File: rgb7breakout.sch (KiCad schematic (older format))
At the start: 8 parts

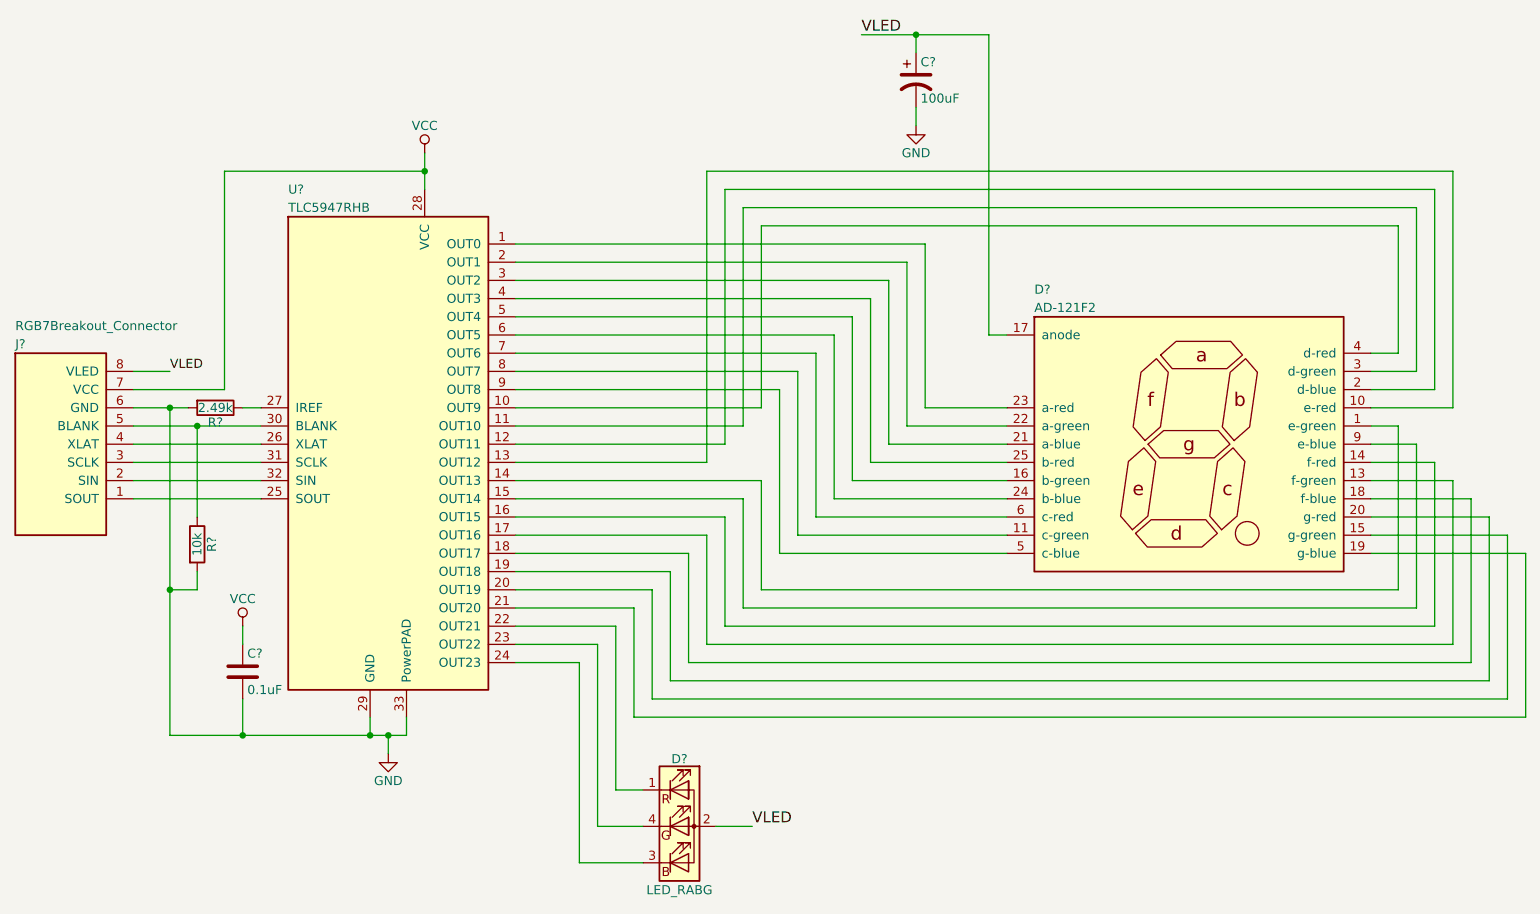
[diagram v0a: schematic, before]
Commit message: annotated components
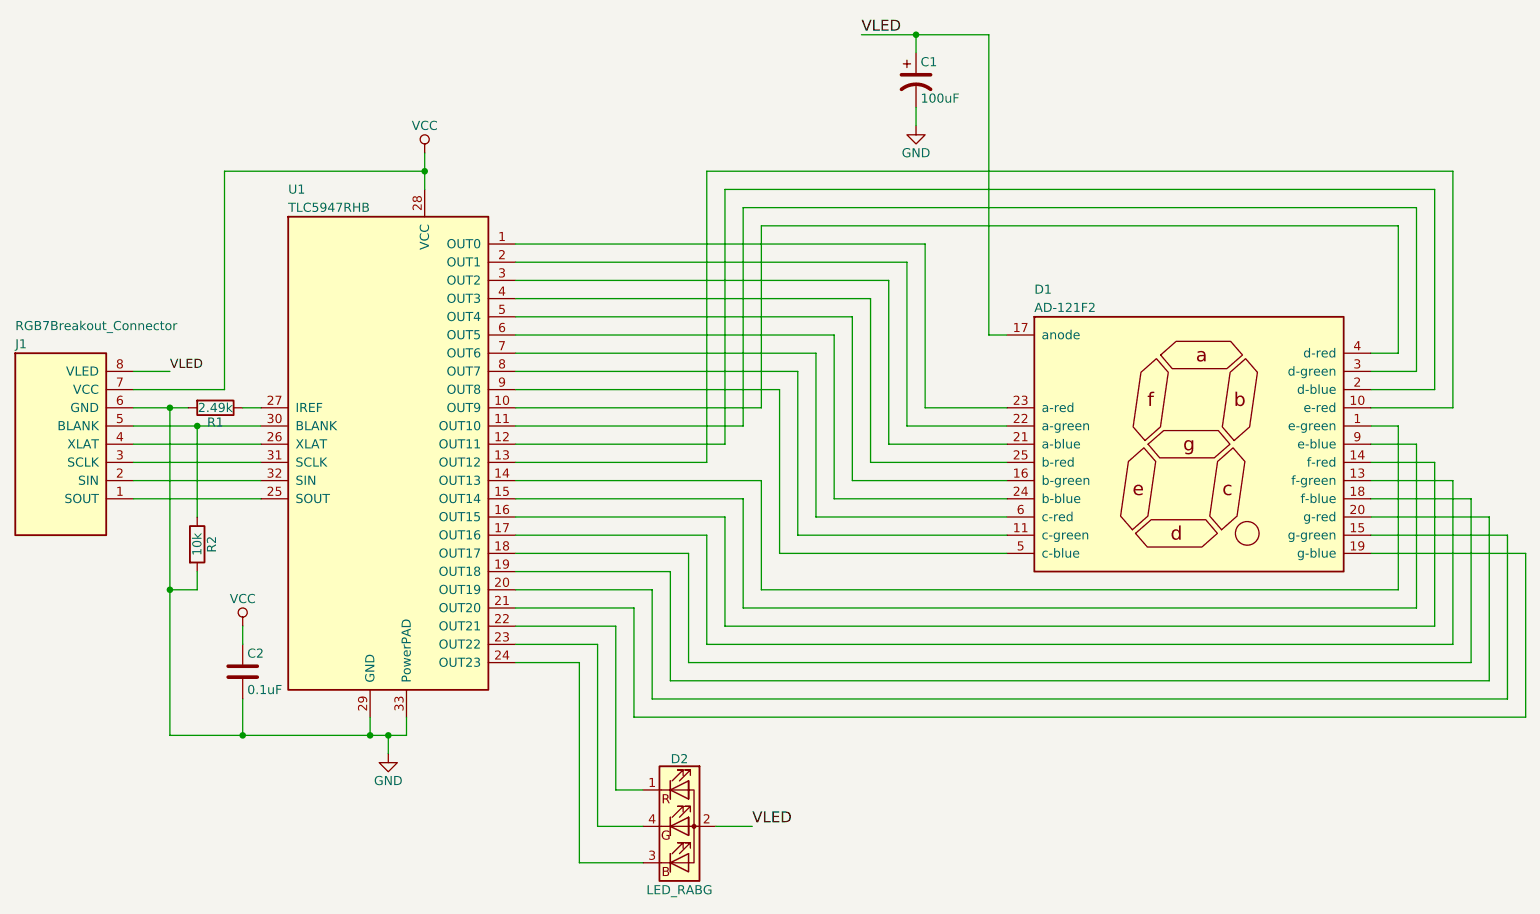
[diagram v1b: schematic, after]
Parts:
- gave numbers to parts that had none: 8
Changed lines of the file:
@@
 $EndDescr
 $Comp
-L AD-121F2 D?
+L AD-121F2 D1
 U 1 1 59B77441
 P 7900 3900
-F 0 "D?" H 7050 4750 50  0000 L CNN
+F 0 "D1" H 7050 4750 50  0000 L CNN
 F 1 "AD-121F2" H 7050 4650 50  0000 L CNN
 F 2 "" H 7900 3900 50  0001 C CNN
@@
 $EndComp
 $Comp
-L LED_RABG D?
+L LED_RABG D2
 U 1 1 59B77822
 P 5100 6000
-F 0 "D?" H 5100 6370 50  0000 C CNN
+F 0 "D2" H 5100 6370 50  0000 C CNN
 F 1 "LED_RABG" H 5100 5650 50  0000 C CNN
 F 2 "" H 5100 5950 50  0001 C CNN
@@
 $EndComp
 $Comp
-L VCC #PWR?
+L VCC #PWR2
 U 1 1 59B778E2
 P 3700 2300
-F 0 "#PWR?" H 3700 2150 50  0001 C CNN
+F 0 "#PWR2" H 3700 2150 50  0001 C CNN
 F 1 "VCC" H 3700 2450 50  0000 C CNN
 F 2 "" H 3700 2300 50  0001 C CNN
@@
 $EndComp
 $Comp
-L GND #PWR?
+L GND #PWR4
 U 1 1 59B77905
 P 3500 5600
-F 0 "#PWR?" H 3500 5350 50  0001 C CNN
+F 0 "#PWR4" H 3500 5350 50  0001 C CNN
 F 1 "GND" H 3500 5450 50  0000 C CNN
 F 2 "" H 3500 5600 50  0001 C CNN
@@
 	5300 6000 5500 6000
 $Comp
-L RGB7Breakout_Connector J?
+L RGB7Breakout_Connector J1
 U 1 1 59B77FB5
 P 1700 3900
-F 0 "J?" H 1450 4450 50  0000 L CNN
+F 0 "J1" H 1450 4450 50  0000 L CNN
 F 1 "RGB7Breakout_Connector" H 1450 4550 50  0000 L CNN
 F 2 "" H 1700 3900 60  0001 C CNN
@@
 Connection ~ 3400 5500
 $Comp
-L R R?
+L R R1
 U 1 1 59B782F7
 P 2550 3700
-F 0 "R?" V 2630 3700 50  0000 C CNN
+F 0 "R1" V 2630 3700 50  0000 C CNN
 F 1 "2.49k" V 2550 3700 50  0000 C CNN
 F 2 "" V 2480 3700 50  0001 C CNN
@@
 	4550 6200 4900 6200
 $Comp
-L CP1 C?
+L CP1 C1
 U 1 1 59B79947
 P 6400 1900
-F 0 "C?" H 6425 2000 50  0000 L CNN
+F 0 "C1" H 6425 2000 50  0000 L CNN
 F 1 "100uF" H 6425 1800 50  0000 L CNN
 F 2 "" H 6400 1900 50  0001 C CNN
@@
 $EndComp
 $Comp
-L VCC #PWR?
+L VCC #PWR3
 U 1 1 59B799AD
 P 2700 4900
-F 0 "#PWR?" H 2700 4750 50  0001 C CNN
+F 0 "#PWR3" H 2700 4750 50  0001 C CNN
 F 1 "VCC" H 2700 5050 50  0000 C CNN
 F 2 "" H 2700 4900 50  0001 C CNN
@@
 Connection ~ 2700 5500
 $Comp
-L C C?
+L C C2
 U 1 1 59B79BCD
 P 2700 5150
-F 0 "C?" H 2725 5250 50  0000 L CNN
+F 0 "C2" H 2725 5250 50  0000 L CNN
 F 1 "0.1uF" H 2725 5050 50  0000 L CNN
 F 2 "" H 2738 5000 50  0001 C CNN
@@
 Connection ~ 6400 1650
 $Comp
-L GND #PWR?
+L GND #PWR1
 U 1 1 59B79DA4
 P 6400 2150
-F 0 "#PWR?" H 6400 1900 50  0001 C CNN
+F 0 "#PWR1" H 6400 1900 50  0001 C CNN
 F 1 "GND" H 6400 2000 50  0000 C CNN
 F 2 "" H 6400 2150 50  0001 C CNN
@@
 	6400 2050 6400 2150
 $Comp
-L R R?
+L R R2
 U 1 1 59B7A418
 P 2450 4450
-F 0 "R?" V 2530 4450 50  0000 C CNN
+F 0 "R2" V 2530 4450 50  0000 C CNN
 F 1 "10k" V 2450 4450 50  0000 C CNN
 F 2 "" V 2380 4450 50  0001 C CNN
@@
 Connection ~ 2300 4700
 $Comp
-L TLC5947RHB U?
+L TLC5947RHB U1
 U 1 1 59B82404
 P 3500 4000
-F 0 "U?" H 2950 5500 50  0000 L CNN
+F 0 "U1" H 2950 5500 50  0000 L CNN
 F 1 "TLC5947RHB" H 2950 5400 50  0000 L CNN
 F 2 "" H 3500 4000 50  0001 C CNN
